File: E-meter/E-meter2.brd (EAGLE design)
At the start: 89.8 x 72.4 mm, 32 parts, among them IC1 LM324N, IC2 7805T

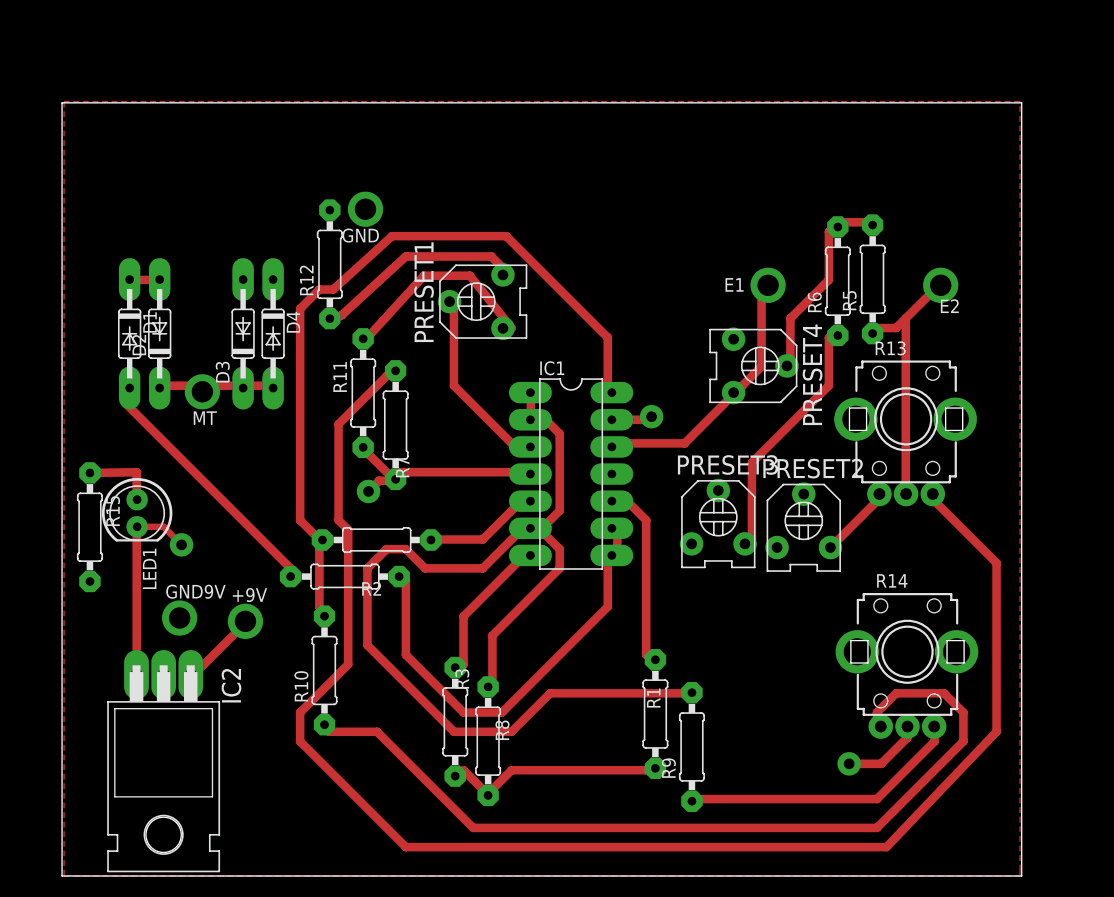
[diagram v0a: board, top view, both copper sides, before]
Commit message: new layout
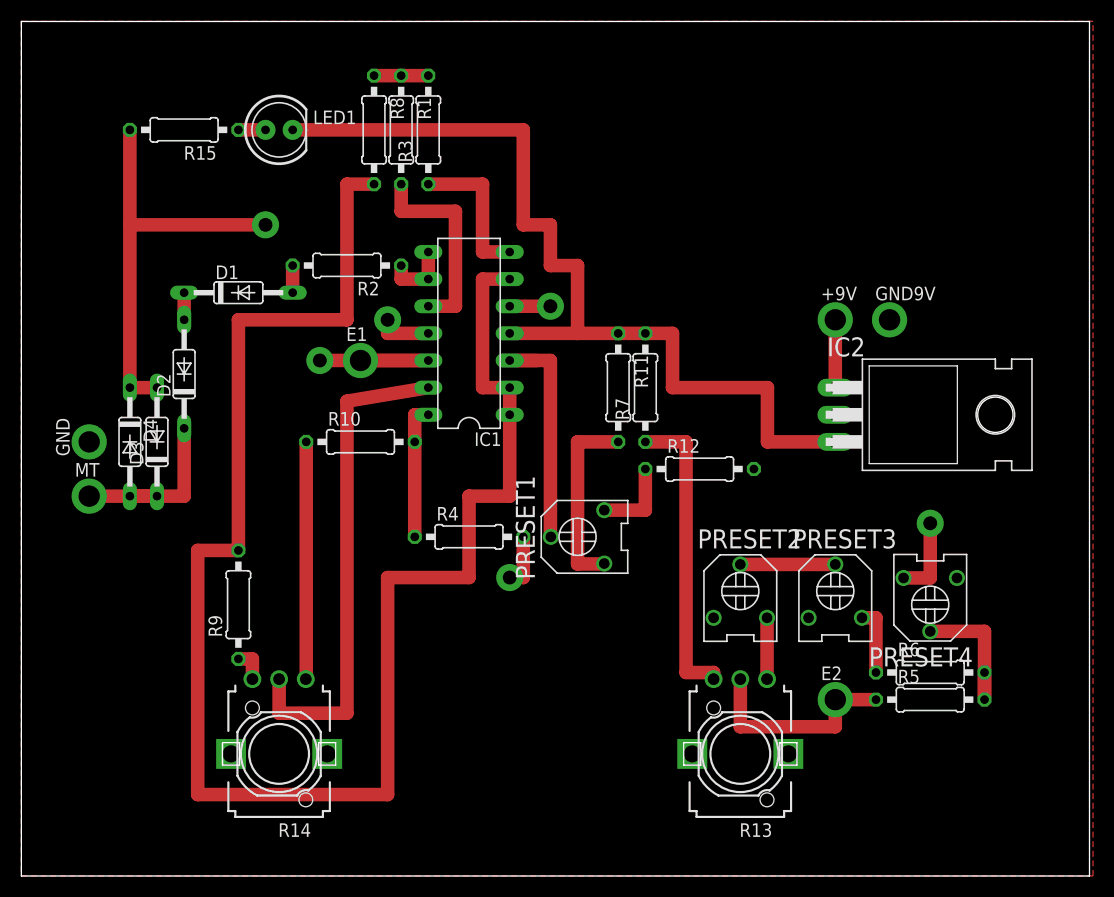
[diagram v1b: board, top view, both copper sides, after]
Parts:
- R13, R14: value POT_US-EVUF2A -> POT_US-EVUF2M; device 4009dist_PWM3_v1:POT_EVUF -> 4009dist_PWM3_v1:POT_EVUFXM
- moved IC2 80.8 mm to (86.4, 43.2), turned to 270 degrees
- moved GND9V 72.1 mm to (81.3, 52.1)
- moved +9V 62.0 mm to (76.2, 52.1)
- moved R1 59.6 mm to (35.6, 69.8), turned to 270 degrees
- moved R14 59.6 mm to (24.1, 11.4), turned to 180 degrees
- moved R8 58.2 mm to (33.0, 69.8), turned to 270 degrees
- moved R3 55.5 mm to (38.1, 69.8), turned to 90 degrees
- moved R9 44.5 mm to (20.3, 25.4)
- moved E2 40.0 mm to (76.2, 16.5), turned to 0 degrees
- moved R5 39.7 mm to (85.1, 16.5), turned to 0 degrees
- moved R12 39.6 mm to (63.5, 38.1), turned to 0 degrees
- moved E1 38.8 mm to (31.8, 48.3), turned to 0 degrees
- moved LED1 38.3 mm to (24.1, 69.8), turned to 0 degrees
- moved R15 38.2 mm to (15.2, 69.8), turned to 180 degrees
- moved R6 37.6 mm to (85.1, 19.1), turned to 0 degrees
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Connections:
- new net N$18: GND9V.1
- net GND: no longer GND9V.1
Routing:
- net N$15: track 137.9 -> 28.6 mm
- net N$4: track 96.7 -> 156.2 mm
- net N$17: track 81.0 -> 22.3 mm
- net N$6: track 70.6 -> 12.7 mm
- net GND: track 0.00 -> 53.3 mm
- net N$14: track 44.0 -> 86.4 mm
- net N$20: track 11.3 -> 46.5 mm
- net N$7: track 41.2 -> 6.35 mm
- net N$21: track 26.4 -> 3.20 mm
- net N$8: track 24.0 -> 2.54 mm
- net N$24: track 23.5 -> 6.43 mm
- net N$22: track 21.0 -> 5.08 mm
- net N$16: track 20.5 -> 7.70 mm
- net N$11: track 11.6 -> 17.8 mm
- net N$12: track 17.4 -> 22.9 mm
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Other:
- board size 89.8 x 72.4 mm -> 100 x 80 mm
